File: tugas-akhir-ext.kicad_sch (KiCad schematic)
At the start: 31 parts, among them J1 Conn_01x02_Socket, J2 Conn_01x02_Pin (solenoid line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, K1 Relay_SPDT, M1 Stepper_Motor_bipolar / Nema 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, M2 Stepper_Motor_bipolar / Nema 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, M3 Stepper_Motor_bipolar / Nema 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, Q1 2N3904, U1 ESP32-DEVKIT-V1, U2 DCDC_StepDown_LM2596, U3 TMC2208_SILENTSTEPSTICK, U4 TMC2208_SILENTSTEPSTICK, U5 TMC2208_SILENTSTEPSTICK

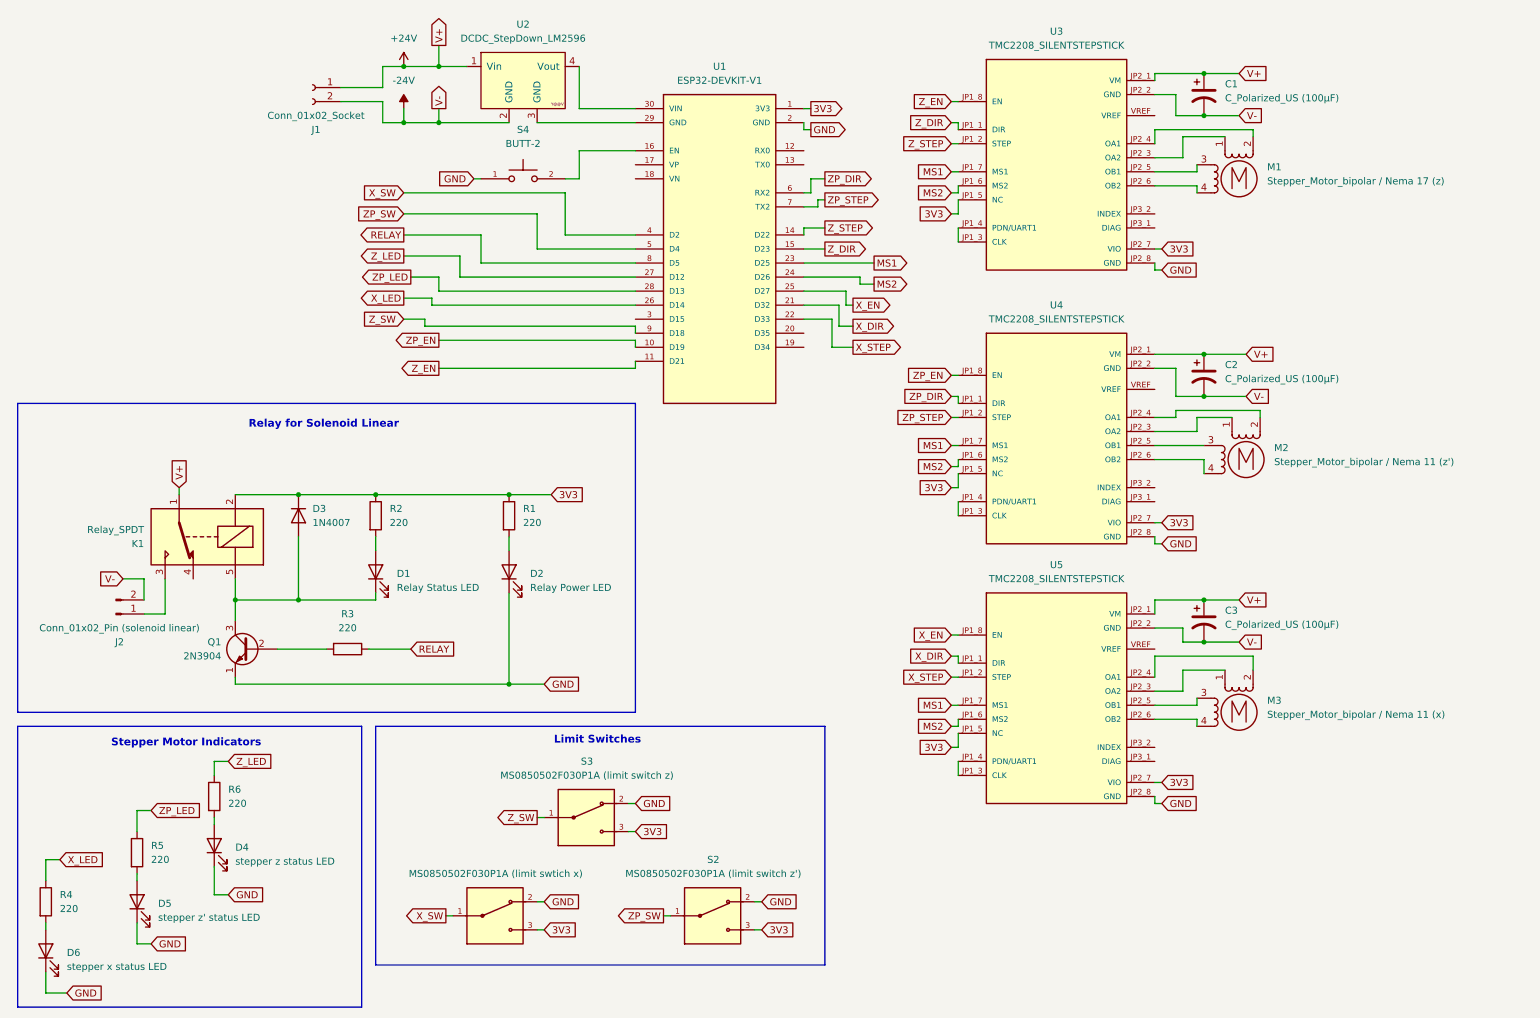
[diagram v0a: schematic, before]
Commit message: minor changes
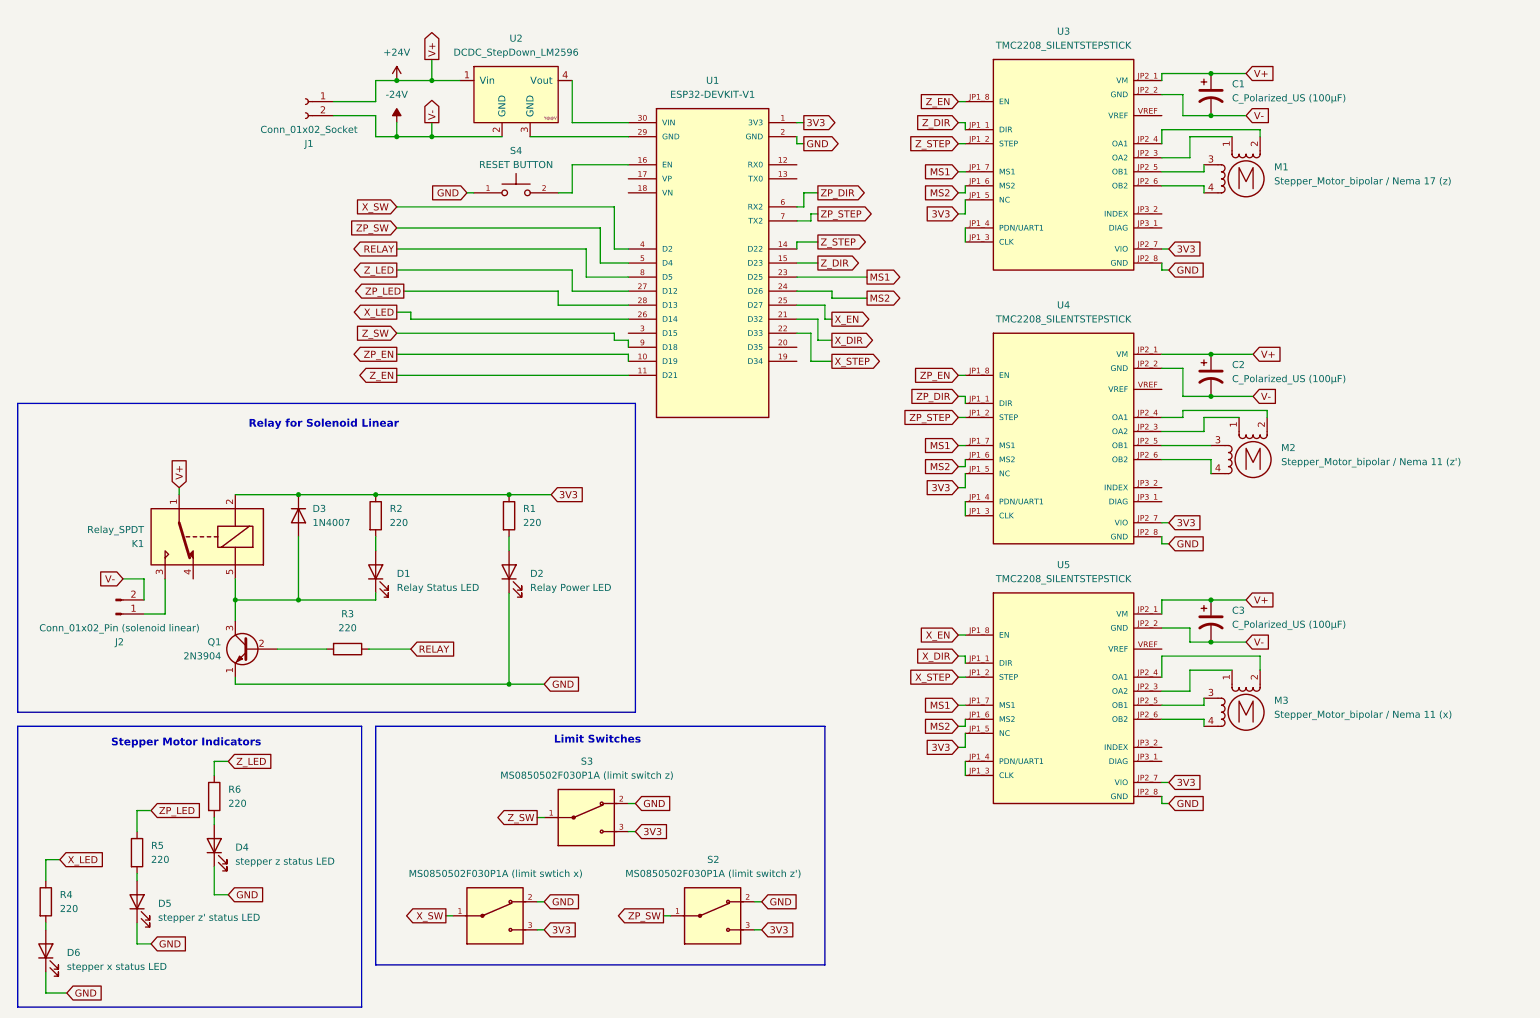
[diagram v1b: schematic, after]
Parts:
- S4: value BUTT-2 -> RESET BUTTON
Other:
- moved on the sheet: C1, C2, C3, J1, M1, M2, M3, S4, U1, U2, U3, U4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
